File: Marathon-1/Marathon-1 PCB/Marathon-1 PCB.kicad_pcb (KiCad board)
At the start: 2 copper layers, 28.5 x 43 mm, 17 parts, among them J1 Conn_01x02_Pin, SW1 SW_Push, U2 XIAO-nRF52840-SMD

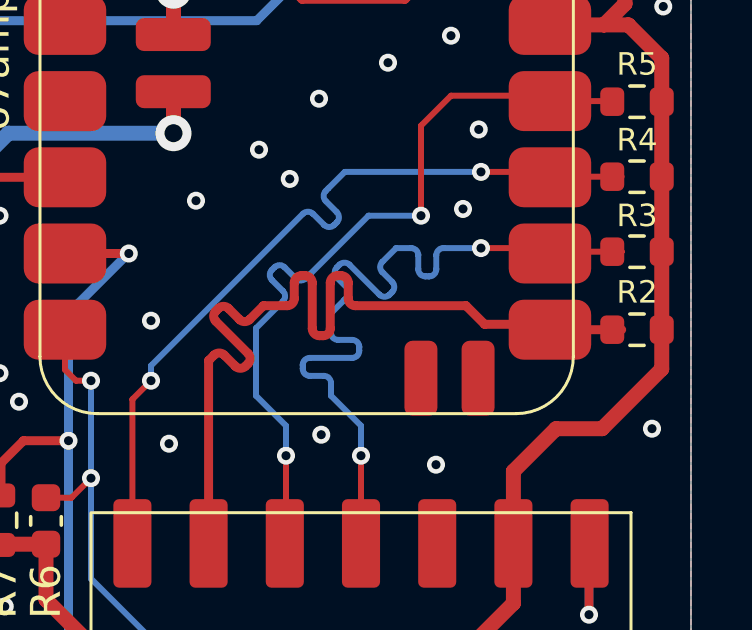
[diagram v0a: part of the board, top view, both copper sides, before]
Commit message: 8
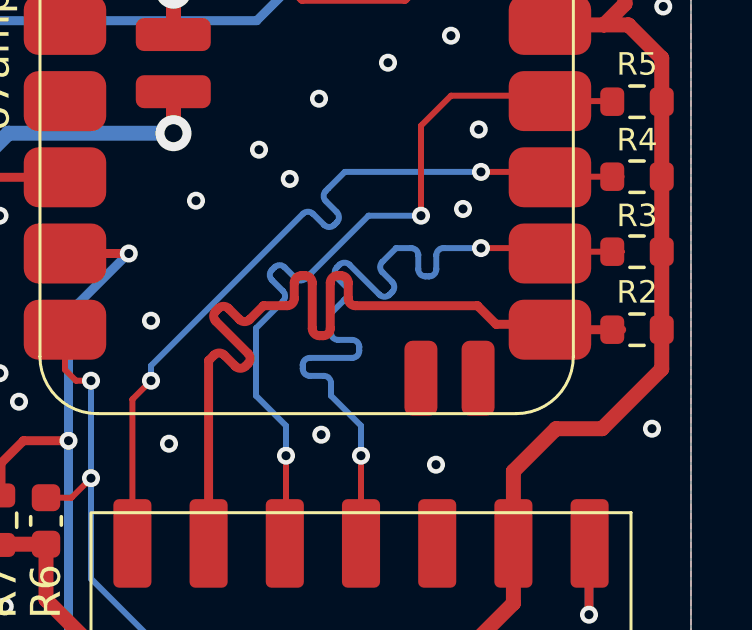
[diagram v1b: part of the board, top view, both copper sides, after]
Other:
- rule pad_to_mask_clearance: 0 -> 0.0508
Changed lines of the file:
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@@
 			(dielectric_constraints no)
 		)
-		(pad_to_mask_clearance 0)
+		(pad_to_mask_clearance 0.0508)
 		(allow_soldermask_bridges_in_footprints no)
 		(tenting front back)
@@
 	)
 	(gr_text ":3"
-		(at 134.425 113.675 0)
+		(at 133.575 113.75 0)
 		(layer "B.SilkS")
 		(effects
@@
 			(polygon
 				(pts
-					(xy 137.584891 94.672732) (xy 137.584891 91.253332) (xy 141.085197 91.253332) (xy 141.085197 94.672732)
+					(xy 136.734891 94.747732) (xy 136.734891 91.328332) (xy 140.235197 91.328332) (xy 140.235197 94.747732)
 				)
 			)
 			(polygon
 				(pts
-					(xy 137.584891 109.425) (xy 137.584891 106.0056) (xy 141.085197 106.0056) (xy 141.085197 109.425)
+					(xy 136.734891 109.5) (xy 136.734891 106.0806) (xy 140.235197 106.0806) (xy 140.235197 109.5)
 				)
 			)
 			(polygon
 				(pts
-					(xy 145.614375 102.781594) (xy 148.688782 102.390806) (xy 149.166778 104.072521) (xy 149.774939 105.284572)
-					(xy 150.490073 106.130774) (xy 151.394478 106.763724) (xy 152.416315 107.144345) (xy 153.59043 107.275662)
-					(xy 154.973071 107.105222) (xy 156.179068 106.608092) (xy 157.252547 105.770516) (xy 158.081234 104.689096)
-					(xy 158.576365 103.460903) (xy 158.747008 102.039706) (xy 158.587076 100.682743) (xy 158.127044 99.532354)
-					(xy 157.363982 98.540928) (xy 156.368987 97.781876) (xy 155.21259 97.323519) (xy 153.846885 97.164009)
-					(xy 152.930205 97.240032) (xy 151.677704 97.505949) (xy 152.018117 94.770429) (xy 152.514235 94.805539)
-					(xy 153.793665 94.689904) (xy 154.96436 94.35075) (xy 156.049651 93.787351) (xy 156.731525 93.214472)
-					(xy 157.214298 92.518682) (xy 157.513991 91.675811) (xy 157.620437 90.645778) (xy 157.489203 89.574046)
-					(xy 157.109767 88.65888) (xy 156.475549 87.862936) (xy 155.654521 87.258092) (xy 154.684067 86.888833)
-					(xy 153.521737 86.759263) (xy 152.370638 86.889283) (xy 151.386894 87.263588) (xy 150.532815 87.88278)
-					(xy 149.862777 88.70478) (xy 149.344147 89.804645) (xy 148.995612 91.253332) (xy 145.922732 90.667149)
-					(xy 146.313235 89.161817) (xy 146.873944 87.887821) (xy 147.596447 86.811356) (xy 148.484228 85.907466)
-					(xy 149.525633 85.179351) (xy 150.685516 84.655078) (xy 151.985778 84.33152) (xy 153.45457 84.219138)
-					(xy 154.798919 84.318877) (xy 156.051079 84.612092) (xy 157.228122 85.096885) (xy 158.304869 85.765917)
-					(xy 159.176495 86.56182) (xy 159.865945 87.491992) (xy 160.377518 88.532879) (xy 160.679442 89.601065)
-					(xy 160.780329 90.712944) (xy 160.682291 91.76669) (xy 160.392927 92.743568) (xy 159.908688 93.662177)
-					(xy 159.254865 94.467747) (xy 158.405702 95.171255) (xy 157.330399 95.774877) (xy 158.729998 96.254562)
-					(xy 159.864983 96.963783) (xy 160.778803 97.907423) (xy 161.44787 99.043349) (xy 161.862956 100.376699)
-					(xy 162.009176 101.955748) (xy 161.857041 103.551013) (xy 161.412484 104.991327) (xy 160.674728 106.310139)
-					(xy 159.618649 107.530591) (xy 158.357964 108.521689) (xy 156.950746 109.229636) (xy 155.368366 109.664739)
-					(xy 153.572112 109.815788) (xy 151.947484 109.68569) (xy 150.514432 109.311253) (xy 149.239701 108.703731)
-					(xy 148.098019 107.857266) (xy 147.130162 106.810421) (xy 146.399439 105.630938) (xy 145.893003 104.297978)
+					(xy 144.764375 102.856594) (xy 147.838782 102.465806) (xy 148.316778 104.147521) (xy 148.924939 105.359572)
+					(xy 149.640073 106.205774) (xy 150.544478 106.838724) (xy 151.566315 107.219345) (xy 152.74043 107.350662)
+					(xy 154.123071 107.180222) (xy 155.329068 106.683092) (xy 156.402547 105.845516) (xy 157.231234 104.764096)
+					(xy 157.726365 103.535903) (xy 157.897008 102.114706) (xy 157.737076 100.757743) (xy 157.277044 99.607354)
+					(xy 156.513982 98.615928) (xy 155.518987 97.856876) (xy 154.36259 97.398519) (xy 152.996885 97.239009)
+					(xy 152.080205 97.315032) (xy 150.827704 97.580949) (xy 151.168117 94.845429) (xy 151.664235 94.880539)
+					(xy 152.943665 94.764904) (xy 154.11436 94.42575) (xy 155.199651 93.862351) (xy 155.881525 93.289472)
+					(xy 156.364298 92.593682) (xy 156.663991 91.750811) (xy 156.770437 90.720778) (xy 156.639203 89.649046)
+					(xy 156.259767 88.73388) (xy 155.625549 87.937936) (xy 154.804521 87.333092) (xy 153.834067 86.963833)
+					(xy 152.671737 86.834263) (xy 151.520638 86.964283) (xy 150.536894 87.338588) (xy 149.682815 87.95778)
+					(xy 149.012777 88.77978) (xy 148.494147 89.879645) (xy 148.145612 91.328332) (xy 145.072732 90.742149)
+					(xy 145.463235 89.236817) (xy 146.023944 87.962821) (xy 146.746447 86.886356) (xy 147.634228 85.982466)
+					(xy 148.675633 85.254351) (xy 149.835516 84.730078) (xy 151.135778 84.40652) (xy 152.60457 84.294138)
+					(xy 153.948919 84.393877) (xy 155.201079 84.687092) (xy 156.378122 85.171885) (xy 157.454869 85.840917)
+					(xy 158.326495 86.63682) (xy 159.015945 87.566992) (xy 159.527518 88.607879) (xy 159.829442 89.676065)
+					(xy 159.930329 90.787944) (xy 159.832291 91.84169) (xy 159.542927 92.818568) (xy 159.058688 93.737177)
+					(xy 158.404865 94.542747) (xy 157.555702 95.246255) (xy 156.480399 95.849877) (xy 157.879998 96.329562)
+					(xy 159.014983 97.038783) (xy 159.928803 97.982423) (xy 160.59787 99.118349) (xy 161.012956 100.451699)
+					(xy 161.159176 102.030748) (xy 161.007041 103.626013) (xy 160.562484 105.066327) (xy 159.824728 106.385139)
+					(xy 158.768649 107.605591) (xy 157.507964 108.596689) (xy 156.100746 109.304636) (xy 154.518366 109.739739)
+					(xy 152.722112 109.890788) (xy 151.097484 109.76069) (xy 149.664432 109.386253) (xy 148.389701 108.778731)
+					(xy 147.248019 107.932266) (xy 146.280162 106.885421) (xy 145.549439 105.705938) (xy 145.043003 104.372978)
 				)
 			)
@@
 	)
 	(segment
-		(start 158.067909 94.203125)
-		(end 156.07 94.203125)
-		(width 0.3)
-		(layer "F.Cu")
-		(net 11)
-	)
-	(segment
 		(start 148.7 93.583125)
 		(end 149.485352 93.583125)
@@
 	)
 	(segment
+		(start 155.833125 93.583125)
+		(end 151.765352 93.583125)
+		(width 0.3)
+		(layer "F.Cu")
+		(net 11)
+	)
+	(segment
 		(start 150.685352 94.583125)
 		(end 150.565352 94.583125)
@@
 	)
 	(segment
-		(start 155.45 93.583125)
-		(end 151.765352 93.583125)
+		(start 148.7 93.583125)
+		(end 148.24038 94.042744)
 		(width 0.3)
 		(layer "F.Cu")
@@
 	)
 	(segment
-		(start 148.7 93.583125)
-		(end 148.24038 94.042744)
+		(start 156.453125 94.203125)
+		(end 155.833125 93.583125)
 		(width 0.3)
 		(layer "F.Cu")
@@
 	)
 	(segment
-		(start 156.07 94.203125)
-		(end 155.45 93.583125)
+		(start 158.067909 94.203125)
+		(end 156.453125 94.203125)
 		(width 0.3)
 		(layer "F.Cu")
